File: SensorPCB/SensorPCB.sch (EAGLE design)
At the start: 31 parts, among them T1 33u

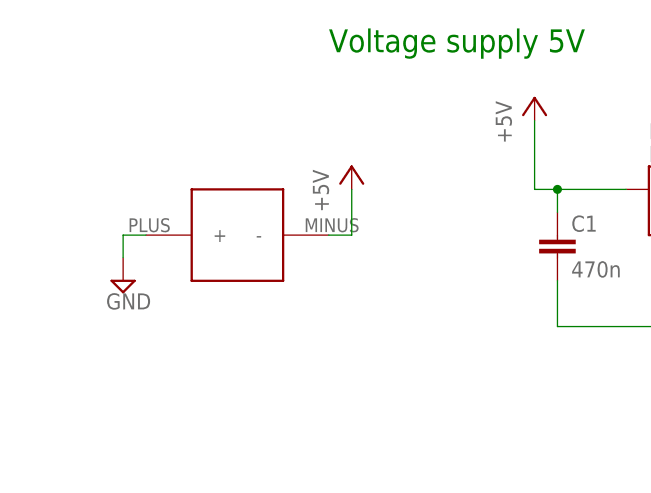
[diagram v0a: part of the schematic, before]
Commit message: closed #1
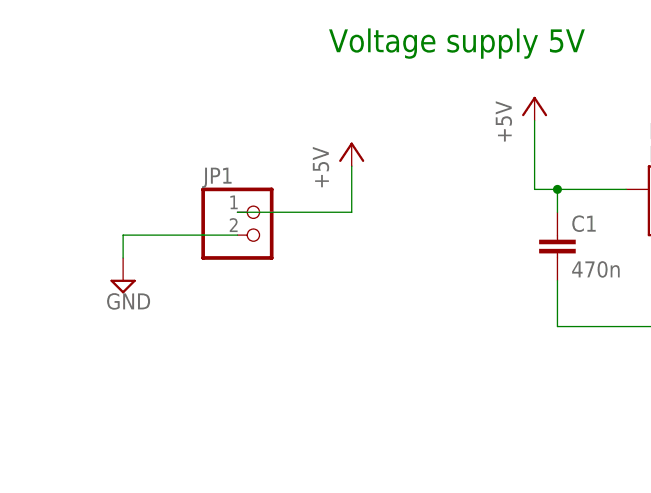
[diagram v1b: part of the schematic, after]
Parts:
- removed U$2: 5V_POWER_SUPPLY, 5V_POWER_SUPPLY:5V_POWER_SUPPLY
- added JP1: (no value), pinhead:PINHD-1X2_2.54-SMD
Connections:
- net +5V: now also JP1.1; no longer U$2.-
- net GND: now also JP1.2; no longer U$2.+
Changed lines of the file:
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@@
 <part name="+3V15" library="supply1" deviceset="+3V3" device=""/>
 <part name="SUPPLY24" library="supply2" deviceset="GND" device=""/>
-<part name="U$2" library="5V_POWER_SUPPLY" deviceset="5V_POWER_SUPPLY" device=""/>
 <part name="P+2" library="supply1" deviceset="+5V" device=""/>
 <part name="SUPPLY25" library="supply2" deviceset="GND" device=""/>
 <part name="R4" library="rcl" deviceset="R-EU_" device="R0805" value="10k"/>
 <part name="+3V7" library="supply1" deviceset="+3V3" device=""/>
+<part name="JP1" library="pinhead" deviceset="PINHD-1X2" device="_2.54-SMD"/>
 </parts>
 <sheets>
@@
 <instance part="+3V15" gate="G$1" x="43.18" y="185.42"/>
 <instance part="SUPPLY24" gate="GND" x="17.78" y="172.72"/>
-<instance part="U$2" gate="G$1" x="30.48" y="223.52"/>
-<instance part="P+2" gate="1" x="43.18" y="231.14"/>
+<instance part="P+2" gate="1" x="43.18" y="233.68"/>
 <instance part="SUPPLY25" gate="GND" x="17.78" y="218.44"/>
 <instance part="R4" gate="G$1" x="294.64" y="223.52" rot="R180"/>
 <instance part="+3V7" gate="G$1" x="287.02" y="223.52" rot="R90"/>
+<instance part="JP1" gate="G$1" x="33.02" y="223.52"/>
 </instances>
 <busses>
@@
 <pinref part="SUPPLY25" gate="GND" pin="GND"/>
 <wire x1="17.78" y1="220.98" x2="17.78" y2="223.52" width="0.1524" layer="91"/>
-<pinref part="U$2" gate="G$1" pin="+"/>
-<wire x1="17.78" y1="223.52" x2="20.32" y2="223.52" width="0.1524" layer="91"/>
+<pinref part="JP1" gate="G$1" pin="2"/>
+<wire x1="17.78" y1="223.52" x2="30.48" y2="223.52" width="0.1524" layer="91"/>
 </segment>
 </net>
@@
 </segment>
 <segment>
-<pinref part="U$2" gate="G$1" pin="-"/>
 <pinref part="P+2" gate="1" pin="+5V"/>
-<wire x1="40.64" y1="223.52" x2="43.18" y2="223.52" width="0.1524" layer="91"/>
-<wire x1="43.18" y1="223.52" x2="43.18" y2="228.6" width="0.1524" layer="91"/>
+<pinref part="JP1" gate="G$1" pin="1"/>
+<wire x1="43.18" y1="226.06" x2="43.18" y2="231.14" width="0.1524" layer="91"/>
+<wire x1="30.48" y1="226.06" x2="43.18" y2="226.06" width="0.1524" layer="91"/>
 </segment>
 </net>
